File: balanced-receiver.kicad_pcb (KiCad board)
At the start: 2 copper layers, 52.5 x 40 mm, 54 parts, among them J1 NC3FAH2, J2 Barrel_Jack_Switch, J3 Screw_Terminal_01x02, J4 Screw_Terminal_01x02, J5 Screw_Terminal_01x02, J6 Screw_Terminal_01x02, J7 Screw_Terminal_01x02, J8 Conn_01x02_Pin, Q1 Q_PMOS_GDS, U1 THAT1240, U2 TPS62932, U3 LM2776

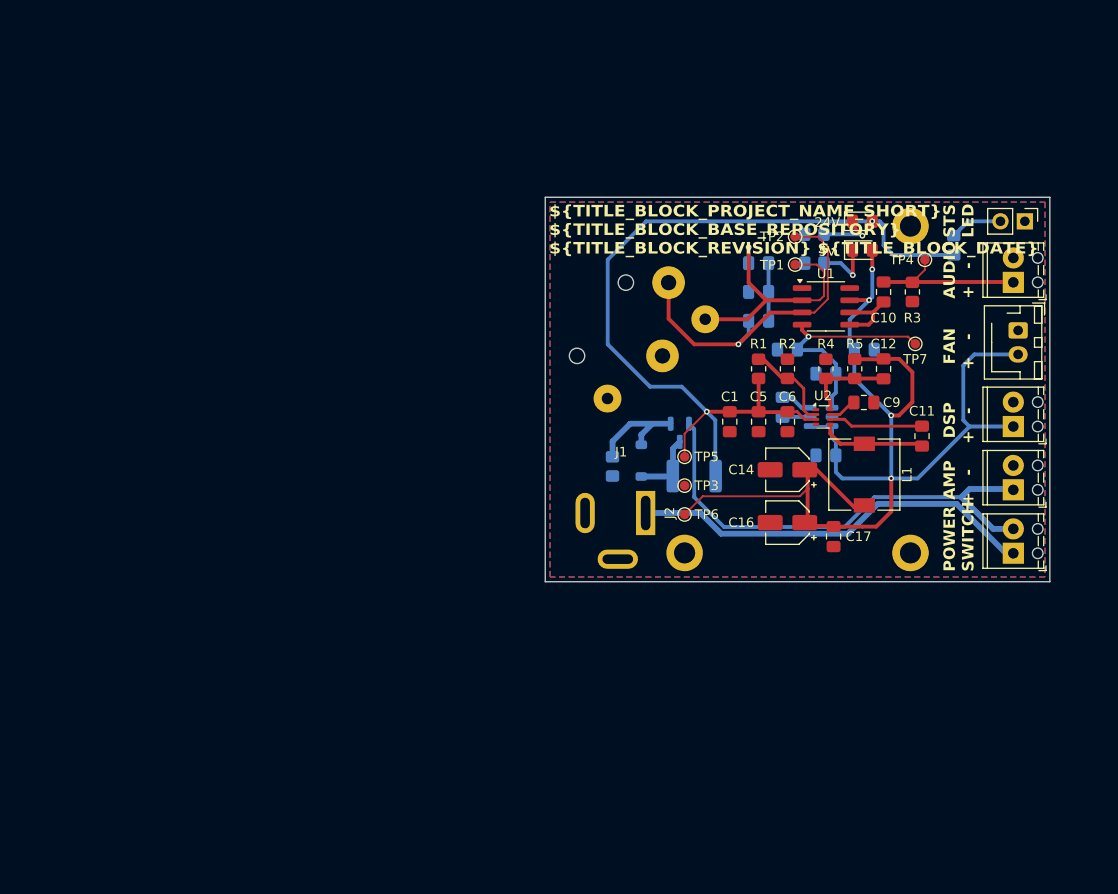
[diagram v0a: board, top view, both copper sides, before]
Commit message: WIP: Converting to schematic
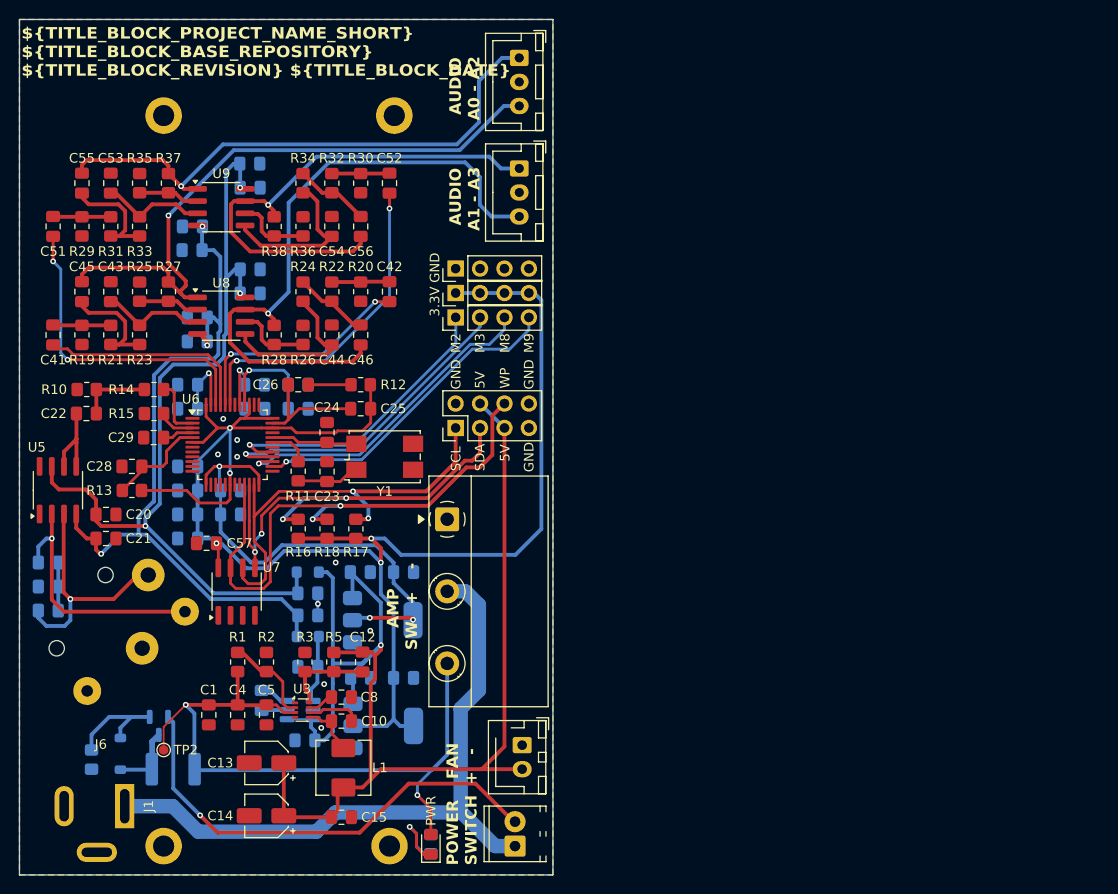
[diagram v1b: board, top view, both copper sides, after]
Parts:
- removed the C10 at (115.3, 57.3)
- removed the C4 at (102.3, 60.3)
- removed the C8 at (105.3, 63.3)
- removed D3: LED, LED_SMD:LED_0805_2012Metric_Pad1.15x1.40mm_HandSolder
- removed the J1 at (92.3, 63.9)
- removed J5: Screw_Terminal_01x02, balanced-receiver:JST_XH_B2B-XH-AM_1x02_P2.50mm_Vertical
- removed J8: Conn_01x02_Pin, Connector_PinHeader_2.54mm:PinHeader_1x02_P2.54mm_Vertical
- removed the R3 at (118.3, 57.3)
- removed the R7 at (122.6, 52.4)
- removed R9: 330Ω, Resistor_SMD:R_0805_2012Metric_Pad1.20x1.40mm_HandSolder
- removed the REF** at (118.1, 50.4)
- removed TP1: Audio+, TestPoint:TestPoint_Pad_D1.0mm
- removed the TP2 at (106.1, 51.5)
- removed TP3, TP7: -5V, TestPoint:TestPoint_Pad_D1.0mm
- removed TP4: AudioOut, TestPoint:TestPoint_Pad_D1.0mm
- removed TP6: +5V, TestPoint:TestPoint_Pad_D1.0mm
- added C17: 47pF, Capacitor_SMD:C_0805_2012Metric_Pad1.18x1.45mm_HandSolder, B.Cu at (28.4, 87.9)
- added C18: 470pF, Capacitor_SMD:C_0805_2012Metric_Pad1.18x1.45mm_HandSolder, B.Cu at (28.4, 85.4)
- added C19: 470pF, Capacitor_SMD:C_0805_2012Metric_Pad1.18x1.45mm_HandSolder, B.Cu at (28.4, 90.4)
- added C20: 100nF, Capacitor_SMD:C_0805_2012Metric_Pad1.18x1.45mm_HandSolder, F.Cu at (34.4, 80.4)
- added C21: 100nF, Capacitor_SMD:C_0805_2012Metric_Pad1.18x1.45mm_HandSolder, F.Cu at (34.4, 82.9)
- added C22: 1uF, Capacitor_SMD:C_0805_2012Metric_Pad1.18x1.45mm_HandSolder, F.Cu at (32.4, 69.9)
- added C23: 22pF, Capacitor_SMD:C_0805_2012Metric_Pad1.18x1.45mm_HandSolder, F.Cu at (57.4, 76.0)
- added C24: 22pF, Capacitor_SMD:C_0805_2012Metric_Pad1.18x1.45mm_HandSolder, F.Cu at (57.4, 71.9)
- added C25: 3.3nF, Capacitor_SMD:C_0805_2012Metric_Pad1.18x1.45mm_HandSolder, F.Cu at (60.9, 69.4)
- added C26: 56nF, Capacitor_SMD:C_0805_2012Metric_Pad1.18x1.45mm_HandSolder, F.Cu at (54.4, 66.9)
- added C27: 10uF, Capacitor_SMD:C_0805_2012Metric_Pad1.18x1.45mm_HandSolder, B.Cu at (42.9, 82.9)
- added C28: 100nF, Capacitor_SMD:C_0805_2012Metric_Pad1.18x1.45mm_HandSolder, F.Cu at (37.1, 75.4)
- added C29: 100nF, Capacitor_SMD:C_0805_2012Metric_Pad1.18x1.45mm_HandSolder, F.Cu at (39.4, 72.4)
- added C30: 100nF, Capacitor_SMD:C_0805_2012Metric_Pad1.18x1.45mm_HandSolder, B.Cu at (42.9, 75.4)
- added C31: 10uF, Capacitor_SMD:C_0805_2012Metric_Pad1.18x1.45mm_HandSolder, B.Cu at (42.9, 69.4)
- added C32: 100nF, Capacitor_SMD:C_0805_2012Metric_Pad1.18x1.45mm_HandSolder, B.Cu at (42.9, 77.9)
- added C33: 100nF, Capacitor_SMD:C_0805_2012Metric_Pad1.18x1.45mm_HandSolder, B.Cu at (42.9, 66.9)
- added C34: 100nF, Capacitor_SMD:C_0805_2012Metric_Pad1.18x1.45mm_HandSolder, B.Cu at (42.9, 80.4)
- added C35: 100nF, Capacitor_SMD:C_0805_2012Metric_Pad1.18x1.45mm_HandSolder, B.Cu at (47.4, 77.9)
- added C36: 10uF, Capacitor_SMD:C_0805_2012Metric_Pad1.18x1.45mm_HandSolder, B.Cu at (47.4, 80.4)
- added C37: 100nF, Capacitor_SMD:C_0805_2012Metric_Pad1.18x1.45mm_HandSolder, B.Cu at (54.4, 66.9)
- added C38: 100nF, Capacitor_SMD:C_0805_2012Metric_Pad1.18x1.45mm_HandSolder, B.Cu at (49.9, 66.9)
- added C39: 10uF, Capacitor_SMD:C_0805_2012Metric_Pad1.18x1.45mm_HandSolder, B.Cu at (54.4, 69.4)
- added C40: 10uF, Capacitor_SMD:C_0805_2012Metric_Pad1.18x1.45mm_HandSolder, B.Cu at (49.9, 69.4)
- added C41: 1uF, Capacitor_SMD:C_0805_2012Metric_Pad1.18x1.45mm_HandSolder, F.Cu at (28.9, 61.8)
- added C42: 1uF, Capacitor_SMD:C_0805_2012Metric_Pad1.18x1.45mm_HandSolder, F.Cu at (63.9, 57.3)
- added C43: 820pF, Capacitor_SMD:C_0805_2012Metric_Pad1.18x1.45mm_HandSolder, F.Cu at (34.9, 57.3)
- added C44: 820pF, Capacitor_SMD:C_0805_2012Metric_Pad1.18x1.45mm_HandSolder, F.Cu at (57.9, 61.8)
- added C45: 680pF, Capacitor_SMD:C_0805_2012Metric_Pad1.18x1.45mm_HandSolder, F.Cu at (31.9, 57.3)
- added C46: 680pF, Capacitor_SMD:C_0805_2012Metric_Pad1.18x1.45mm_HandSolder, F.Cu at (60.9, 61.8)
- added C47: 100nF, Capacitor_SMD:C_0805_2012Metric_Pad1.18x1.45mm_HandSolder, B.Cu at (49.4, 43.9)
- added C48: 100nF, Capacitor_SMD:C_0805_2012Metric_Pad1.18x1.45mm_HandSolder, B.Cu at (43.4, 50.5)
- added C49: 100nF, Capacitor_SMD:C_0805_2012Metric_Pad1.18x1.45mm_HandSolder, B.Cu at (49.4, 57.4)
- added C50: 100nF, Capacitor_SMD:C_0805_2012Metric_Pad1.18x1.45mm_HandSolder, B.Cu at (43.9, 62.4)
- added C51: 1uF, Capacitor_SMD:C_0805_2012Metric_Pad1.18x1.45mm_HandSolder, F.Cu at (28.9, 50.5)
- added C52: 1uF, Capacitor_SMD:C_0805_2012Metric_Pad1.18x1.45mm_HandSolder, F.Cu at (63.9, 46.0)
- added C53: 820pF, Capacitor_SMD:C_0805_2012Metric_Pad1.18x1.45mm_HandSolder, F.Cu at (34.9, 46.0)
- added C54: 820pF, Capacitor_SMD:C_0805_2012Metric_Pad1.18x1.45mm_HandSolder, F.Cu at (57.9, 50.5)
- added C55: 680pF, Capacitor_SMD:C_0805_2012Metric_Pad1.18x1.45mm_HandSolder, F.Cu at (31.9, 46.0)
- added C56: 680pF, Capacitor_SMD:C_0805_2012Metric_Pad1.18x1.45mm_HandSolder, F.Cu at (60.9, 50.5)
- added C57: 100nF, Capacitor_SMD:C_0805_2012Metric_Pad1.18x1.45mm_HandSolder, F.Cu at (44.9, 83.4)
- added C58: 10uF, Capacitor_SMD:C_0805_2012Metric_Pad1.18x1.45mm_HandSolder, B.Cu at (55.4, 88.6)
- added C59: 10uF, Capacitor_SMD:C_0805_2012Metric_Pad1.18x1.45mm_HandSolder, B.Cu at (55.4, 90.9)
- added C6: 10uF, Capacitor_SMD:C_0805_2012Metric_Pad1.18x1.45mm_HandSolder, B.Cu at (65.4, 97.4)
- added C60: 10uF, Capacitor_SMD:C_0805_2012Metric_Pad1.18x1.45mm_HandSolder, B.Cu at (49.4, 46.4)
- added C61: 10uF, Capacitor_SMD:C_0805_2012Metric_Pad1.18x1.45mm_HandSolder, B.Cu at (43.9, 59.9)
- added C62: 10uF, Capacitor_SMD:C_0805_2012Metric_Pad1.18x1.45mm_HandSolder, B.Cu at (43.4, 52.9)
- added C63: 10uF, Capacitor_SMD:C_0805_2012Metric_Pad1.18x1.45mm_HandSolder, B.Cu at (49.4, 54.9)
- added J10: Conn_01x03_Pin, Connector_JST:JST_XH_B3B-XH-A_1x03_P2.50mm_Vertical, F.Cu at (77.4, 32.9)
- added J11: Conn_01x04_Pin, Connector_PinHeader_2.54mm:PinHeader_1x04_P2.54mm_Vertical, F.Cu at (70.8, 59.9)
- added J12: Conn_01x04_Pin, Connector_PinHeader_2.54mm:PinHeader_1x04_P2.54mm_Vertical, F.Cu at (70.8, 57.4)
- added J13: Conn_01x04_Pin, Connector_PinHeader_2.54mm:PinHeader_1x04_P2.54mm_Vertical, F.Cu at (70.8, 54.9)
- added J3: Screw_Terminal_01x02, balanced-receiver:JST_XH_B2B-XH-AM_1x02_P2.50mm_Vertical, F.Cu at (77.7, 104.4)
- added J9: Conn_01x03_Pin, Connector_JST:JST_XH_B3B-XH-A_1x03_P2.50mm_Vertical, F.Cu at (77.4, 44.4)
- added L2: 1uH, Inductor_SMD:L_0805_2012Metric_Pad1.05x1.20mm_HandSolder, B.Cu at (55.4, 86.4)
- added L3: 1uH, Inductor_SMD:L_0805_2012Metric_Pad1.05x1.20mm_HandSolder, B.Cu at (55.4, 93.1)
- added R10: 10kΩ, Resistor_SMD:R_0805_2012Metric_Pad1.20x1.40mm_HandSolder, F.Cu at (32.4, 67.4)
- added R11: 100Ω, Resistor_SMD:R_0805_2012Metric_Pad1.20x1.40mm_HandSolder, F.Cu at (54.4, 75.9)
- added R12: 475Ω, Resistor_SMD:R_0805_2012Metric_Pad1.20x1.40mm_HandSolder, F.Cu at (60.9, 66.9)
- added R13: 10k, Resistor_SMD:R_0805_2012Metric_Pad1.20x1.40mm_HandSolder, F.Cu at (37.1, 77.9)
- added R14: 7kΩ, Resistor_SMD:R_0805_2012Metric_Pad1.20x1.40mm_HandSolder, F.Cu at (39.4, 67.4)
- added R15: 18kΩ, Resistor_SMD:R_0805_2012Metric_Pad1.20x1.40mm_HandSolder, F.Cu at (39.4, 69.9)
- added R16: 2.2kΩ, Resistor_SMD:R_0805_2012Metric_Pad1.20x1.40mm_HandSolder, F.Cu at (54.4, 81.9)
- added R17: 2.2kΩ, Resistor_SMD:R_0805_2012Metric_Pad1.20x1.40mm_HandSolder, F.Cu at (60.4, 81.9)
- added R18: 10kΩ, Resistor_SMD:R_0805_2012Metric_Pad1.20x1.40mm_HandSolder, F.Cu at (57.4, 81.9)
- added R19: 10kΩ, Resistor_SMD:R_0805_2012Metric_Pad1.20x1.40mm_HandSolder, F.Cu at (31.9, 61.8)
- added R20: 10kΩ, Resistor_SMD:R_0805_2012Metric_Pad1.20x1.40mm_HandSolder, F.Cu at (60.9, 57.3)
- added R21: 6.2kΩ, Resistor_SMD:R_0805_2012Metric_Pad1.20x1.40mm_HandSolder, F.Cu at (34.9, 61.8)
- added R22: 6.2kΩ, Resistor_SMD:R_0805_2012Metric_Pad1.20x1.40mm_HandSolder, F.Cu at (57.9, 57.3)
- added R23: 8.2kΩ, Resistor_SMD:R_0805_2012Metric_Pad1.20x1.40mm_HandSolder, F.Cu at (37.9, 61.8)
- added R24: 8.2kΩ, Resistor_SMD:R_0805_2012Metric_Pad1.20x1.40mm_HandSolder, F.Cu at (54.9, 57.3)
- added R25: 10kΩ, Resistor_SMD:R_0805_2012Metric_Pad1.20x1.40mm_HandSolder, F.Cu at (37.9, 57.3)
- added R26: 10kΩ, Resistor_SMD:R_0805_2012Metric_Pad1.20x1.40mm_HandSolder, F.Cu at (54.9, 61.8)
- added R27: 10kΩ, Resistor_SMD:R_0805_2012Metric_Pad1.20x1.40mm_HandSolder, F.Cu at (40.9, 57.3)
- added R28: 10kΩ, Resistor_SMD:R_0805_2012Metric_Pad1.20x1.40mm_HandSolder, F.Cu at (51.9, 61.8)
- added R29: 10kΩ, Resistor_SMD:R_0805_2012Metric_Pad1.20x1.40mm_HandSolder, F.Cu at (31.9, 50.5)
- added R30: 10kΩ, Resistor_SMD:R_0805_2012Metric_Pad1.20x1.40mm_HandSolder, F.Cu at (60.9, 46.0)
- added R31: 6.2kΩ, Resistor_SMD:R_0805_2012Metric_Pad1.20x1.40mm_HandSolder, F.Cu at (34.9, 50.5)
- added R32: 6.2kΩ, Resistor_SMD:R_0805_2012Metric_Pad1.20x1.40mm_HandSolder, F.Cu at (57.9, 46.0)
- added R33: 8.2kΩ, Resistor_SMD:R_0805_2012Metric_Pad1.20x1.40mm_HandSolder, F.Cu at (37.9, 50.5)
- added R34: 8.2kΩ, Resistor_SMD:R_0805_2012Metric_Pad1.20x1.40mm_HandSolder, F.Cu at (54.9, 46.0)
- added R35: 10kΩ, Resistor_SMD:R_0805_2012Metric_Pad1.20x1.40mm_HandSolder, F.Cu at (37.9, 46.0)
- added R36: 10kΩ, Resistor_SMD:R_0805_2012Metric_Pad1.20x1.40mm_HandSolder, F.Cu at (54.9, 50.5)
- added R37: 10kΩ, Resistor_SMD:R_0805_2012Metric_Pad1.20x1.40mm_HandSolder, F.Cu at (40.9, 46.0)
- added R38: 10kΩ, Resistor_SMD:R_0805_2012Metric_Pad1.20x1.40mm_HandSolder, F.Cu at (51.9, 50.5)
- added REF**: MountingHole_2.2mm_M2_DIN965_Pad, MountingHole:MountingHole_2.2mm_M2_DIN965_Pad, F.Cu at (64.4, 38.9)
- added REF**: MountingHole_2.2mm_M2_DIN965_Pad, MountingHole:MountingHole_2.2mm_M2_DIN965_Pad, F.Cu at (40.4, 38.9)
- added U2: LM1117DT-1.8, Package_TO_SOT_SMD:SOT-223-3_TabPin2, B.Cu at (63.2, 91.4)
- added U5: THAT1240, Package_SO:SOIC-8_3.9x4.9mm_P1.27mm, F.Cu at (29.4, 77.9)
- added U6: ADAU1701, Package_QFP:LQFP-48_7x7mm_P0.5mm, F.Cu at (47.6, 73.2)
- added U7: 24LC256, Package_SO:SOIC-8_3.9x4.9mm_P1.27mm, F.Cu at (48.0, 88.5)
- added U8: OPA1612AxD, Package_SO:SOIC-8_3.9x4.9mm_P1.27mm, F.Cu at (46.4, 59.8)
- added U9: OPA1612AxD, Package_SO:SOIC-8_3.9x4.9mm_P1.27mm, F.Cu at (46.4, 48.5)
- added Y1: 12.288 MHz, balanced-receiver:Crystal_SMD_7050-4Pin_7.0x5.0mm, F.Cu at (63.4, 74.4)
- C2: value 47pF -> 10uF
- C3: value 470pF -> 10uF
- C7: value 100nF -> 10uF
- J2: renamed from J3; footprint TerminalBlock_Phoenix:TerminalBlock_Phoenix_MPT-0,5-2-2.54_1x02_P2.54mm_Horizontal -> balanced-receiver:TerminalBlock_Phoenix_MPT-0,5-2-2.54_1x02_P2.54mm_Horizontal
- J4: value Screw_Terminal_01x02 -> Screw_Terminal_01x03; footprint TerminalBlock_Phoenix:TerminalBlock_Phoenix_MPT-0,5-2-2.54_1x02_P2.54mm_Horizontal -> balanced-receiver:TerminalBlock_1x03_P7.50mm_Horizontal
- J6: value Screw_Terminal_01x02 -> NC3FAH2; footprint TerminalBlock_Phoenix:TerminalBlock_Phoenix_MPT-0,5-2-2.54_1x02_P2.54mm_Horizontal -> balanced-receiver:Jack_XLR_Neutrik_NC3FAH2_Horizontal
- J7: value Screw_Terminal_01x02 -> Conn_02x04_Odd_Even; footprint TerminalBlock_Phoenix:TerminalBlock_Phoenix_MPT-0,5-2-2.54_1x02_P2.54mm_Horizontal -> Connector_PinHeader_2.54mm:PinHeader_2x04_P2.54mm_Vertical
- L1: footprint balanced-receiver:L_7.3x7.3_H4.5 -> Inductor_SMD:L_APV_APH0530
- U1: value THAT1240 -> LM1117DT-3.3; footprint Package_SO:SOIC-8_3.9x4.9mm_P1.27mm -> Package_TO_SOT_SMD:SOT-223-3_TabPin2; moved to B.Cu
- U4: renamed from U3; footprint Package_TO_SOT_SMD:SOT-23-6 -> Package_TO_SOT_SMD:SOT-23-6_Handsoldering
- moved J6 93.5 mm to (38.2, 94.4), turned to 180 degrees
- moved D2 78.9 mm to (68.2, 114.8), turned to 90 degrees
- moved R7 75.0 mm to (68.2, 114.7), turned to 90 degrees
- moved C10 67.3 mm to (58.9, 101.9), turned to 180 degrees
- moved U1 63.5 mm to (63.3, 102.4)
- moved C8 62.4 mm to (58.9, 99.4)
- moved C1 62.2 mm to (45.1, 101.3)
- moved C11 62.2 mm to (50.6, 99.8)
- moved C12 62.2 mm to (61.1, 95.8)
- moved C13 62.2 mm to (51.1, 106.3)
- moved C14 62.2 mm to (51.1, 111.8)
- moved C4 62.2 mm to (48.1, 101.3)
- moved C5 62.2 mm to (51.1, 101.3)
- moved D1 62.2 mm to (35.9, 105.3)
- moved F1 62.2 mm to (41.4, 106.9)
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- renumbered C11 to C10, C15 to C11, C14 to C13, C16 to C14, C17 to C15, C18 to C16, C5 to C4, C6 to C5, C9 to C8, C13 to C9, J2 to J1, R4 to R3, R6 to R4, R8 to R7, TP5 to TP2, U2 to U3
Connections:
- C16 pad 1: -5V -> Net-(U4-VOUT)
- C2 pad 2: Net-(C2-Pad2) -> +5V
- C3 pad 1: /Audio- -> GND
- C3 pad 2: Net-(C2-Pad2) -> +5V
- C7 pad 1: +5V -> GND
- C7 pad 2: GND -> +1.8V
- J1 pad 1: Net-(J3-Pin_1) -> VCC_UN
- J2 pad 1: Net-(J3-Pin_1) -> VCC_UN
- J4 pad 1: VCC -> GND
- J4 pad 2: GND -> VCC_UN
- J6 pad 1: +5V -> GND
- J6 pad 2: GND -> /analog_input/Audio+
- J7 pad 1: /AudioOut -> /adau_1701/SCL
- U1 pad 2: /Audio- -> +3.3V
- U1 pad 3: /Audio+ -> +5V
- U4 pad 1: -5V -> Net-(U4-VOUT)
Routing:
- net +3.3V: track 0.00 -> 175.0 mm, vias 0 -> 5
- net +5V_ANALOG: track 0.00 -> 87.1 mm, vias 0 -> 3
- net VCC_UN: track 0.00 -> 70.0 mm
- net /analog_output/AUDIO_OUT_1: track 0.00 -> 66.3 mm, vias 0 -> 1
- net /analog_output/AUDIO_OUT_0: track 0.00 -> 65.1 mm, vias 0 -> 1
- net /adau_1701/WP: track 0.00 -> 59.1 mm, vias 0 -> 2
- net /analog_output/AUDIO_OUT_2: track 0.00 -> 58.1 mm, vias 0 -> 1
- net -5V: track 23.6 -> 79.7 mm, vias 1 -> 3
- net /analog_output/AUDIO_OUT_3: track 0.00 -> 52.7 mm, vias 0 -> 1
- net /adau_1701/SDA: track 0.00 -> 50.1 mm, vias 0 -> 4
- net +1.8V: track 0.00 -> 49.3 mm, vias 0 -> 3
- net /adau_1701/SCL: track 0.00 -> 45.8 mm, vias 0 -> 2
- net Net-(J3-Pin_1): track 42.5 -> 0.00 mm
- net /Audio+: track 35.6 -> 0.00 mm, vias 1 -> 0
- net ADAU_AUDIO_OUTPUT_3: track 0.00 -> 34.5 mm, vias 0 -> 2
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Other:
- board size 52.5 x 40 mm -> 55.5 x 89 mm
- board text added: "3.3V"
- board text added: "AMP SW + -"
- board text added: "AUDIO A0 - A2"
- board text added: "AUDIO A1 - A3"
- board text added: "GND"
- board text added: "M2"
- board text added: "M3"
- board text added: "M8"
- board text added: "M9"
- board text added: "PWR"
- board text added: "SCL"
- board text added: "SDA"
- board text added: "WP"
- board text added: "{ "ViaStitching": "0.2", "stitch_zone_0": { "HSpacing": "5", "VSpacing": "5", "HOffset": "0", "VOffset": "0", "Clearance": "0", "Randomize": false } }"
- board text removed: "24V"
- board text removed: "AMP + -"
- board text removed: "AUDIO + -"
- board text removed: "DSP + -"
- board text removed: "STS LED"
- board text removed: "{ "ViaStitching": "0.2", "stitch_zone_0": { "HSpacing": "5", "VSpacing": "5", "Clearance": "0", "Randomize": false }, "stitch_zone_1": { "HSpacing": "5", "VSpacing": "5", "Clearance": "0", "Randomize": false } }"
